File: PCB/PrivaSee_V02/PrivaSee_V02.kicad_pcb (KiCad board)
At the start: 4 copper layers, 73.8 x 90 mm, 33 parts, among them J1 RFPC-SMA27-F, J2 Batt_Solder_Point, J3 Conn_02x06_Odd_Even, J4 VOUT_TEST, J5 GND_TEST, J6 IR_TEST, J7 RF_TEST, SW1 Switch, SW2 SW_Push, U2 LM358, U3 254, U4 DFR0568, U6 ESP32-C5-DevKitC-1

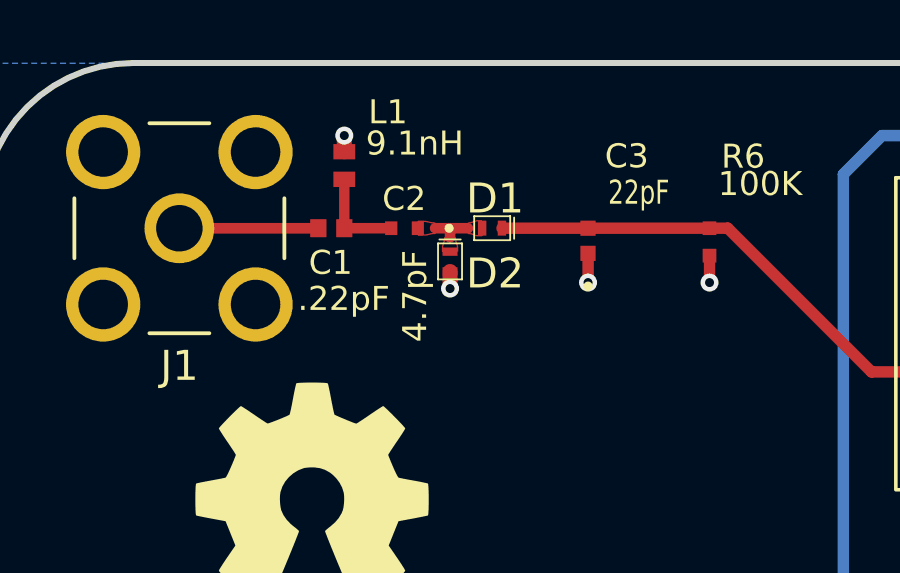
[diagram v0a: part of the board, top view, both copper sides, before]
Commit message: more trace changes
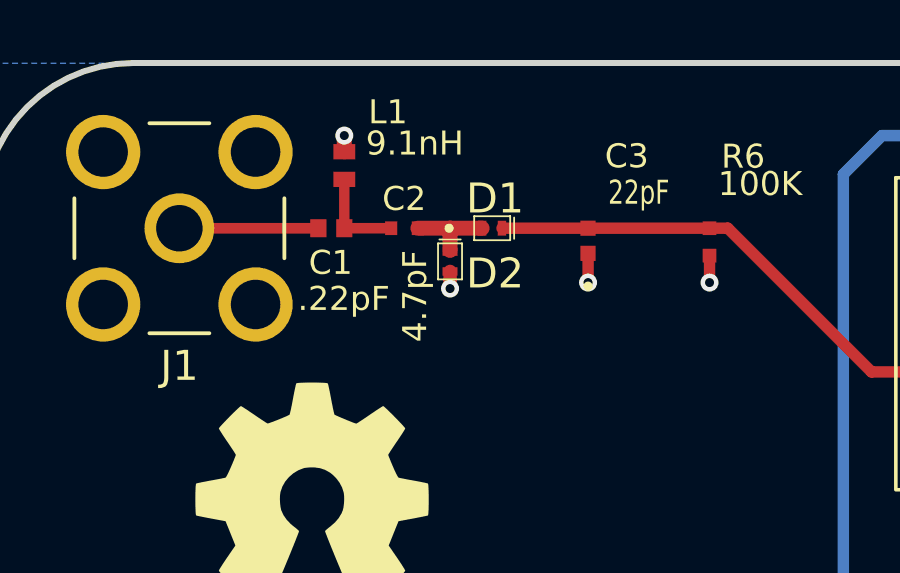
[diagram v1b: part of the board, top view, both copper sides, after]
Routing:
- net Net-(D1-A): track 1.41 -> 2.88 mm
- removed copper zone on F.Cu, net Net-(D1-A)
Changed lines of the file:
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@@
 	)
 	(segment
-		(start 81.6 27.4)
+		(start 81.6 27.0882)
+		(end 82.67 27.0882)
+		(width 0.5)
+		(layer "F.Cu")
+		(net "Net-(D1-A)")
+	)
+	(segment
+		(start 81.6 27.0882)
+		(end 81.6 27.83)
+		(width 0.5)
+		(layer "F.Cu")
+		(net "Net-(D1-A)")
+	)
+	(segment
+		(start 80.527284 27.0882)
 		(end 81.6 27.0882)
-		(width 0.35)
-		(layer "F.Cu")
-		(net "Net-(D1-A)")
-	)
-	(segment
-		(start 81.1 27.0882)
-		(end 81.6 27.0882)
-		(width 0.35)
-		(layer "F.Cu")
-		(net "Net-(D1-A)")
-	)
-	(segment
-		(start 81.6 27.0882)
-		(end 82.2 27.0882)
-		(width 0.35)
+		(width 0.5)
 		(layer "F.Cu")
 		(net "Net-(D1-A)")
@@
 		(start 81.6 29.1)
 		(end 81.6 28.53)
-		(width 0.5)
+		(width 0.45)
 		(layer "F.Cu")
 		(net "GND")
@@
 	)
 	(zone
-		(net "Net-(D1-A)")
-		(layer "F.Cu")
-		(hatch edge 0.5)
-		(priority 17540)
-		(connect_pads yes
-			(clearance 0)
-		)
-		(min_thickness 0.0254)
-		(fill yes
-			(thermal_gap 0.5)
-			(thermal_bridge_width 0.5)
-			(island_removal_mode 0)
-		)
-		(polygon
-			(pts
-				(xy 81.6 27.37375) (xy 81.425 27.3972) (xy 81.4229 27.444513) (xy 81.4172 27.48503) (xy 81.408799 27.520128)
-				(xy 81.3986 27.551189) (xy 81.3875 27.579591) (xy 81.3764 27.606713) (xy 81.3662 27.633936) (xy 81.3578 27.662638)
-				(xy 81.3521 27.6942) (xy 81.35 27.73) (xy 81.35 27.87) (xy 81.6 27.9) (xy 81.85 27.87) (xy 81.85 27.73)
-				(xy 81.8479 27.6942) (xy 81.8422 27.662638) (xy 81.833799 27.633936) (xy 81.8236 27.606713) (xy 81.8125 27.579591)
-				(xy 81.8014 27.551189) (xy 81.7912 27.520128) (xy 81.7828 27.48503) (xy 81.7771 27.444513) (xy 81.775 27.3972)
-			)
-		)
-	)
-	(zone
-		(net "Net-(D1-A)")
-		(layer "F.Cu")
-		(hatch edge 0.5)
-		(priority 17540)
-		(connect_pads yes
-			(clearance 0)
-		)
-		(min_thickness 0.0254)
-		(fill yes
-			(thermal_gap 0.5)
-			(thermal_bridge_width 0.5)
-			(island_removal_mode 0)
-		)
-		(polygon
-			(pts
-				(xy 82.17375 27.0882) (xy 82.1972 27.2632) (xy 82.244513 27.2653) (xy 82.28503 27.271) (xy 82.320128 27.279399)
-				(xy 82.351189 27.2896) (xy 82.379591 27.3007) (xy 82.406713 27.3118) (xy 82.433936 27.321999) (xy 82.462638 27.3304)
-				(xy 82.4942 27.3361) (xy 82.53 27.3382) (xy 82.67 27.3382) (xy 82.7 27.0882) (xy 82.67 26.8382)
-				(xy 82.53 26.8382) (xy 82.4942 26.8403) (xy 82.462638 26.846) (xy 82.433936 26.854399) (xy 82.406713 26.8646)
-				(xy 82.379591 26.8757) (xy 82.351189 26.8868) (xy 82.320128 26.896999) (xy 82.28503 26.9054) (xy 82.244513 26.9111)
-				(xy 82.1972 26.9132)
-			)
-		)
-	)
-	(zone
-		(net "Net-(D1-A)")
-		(layer "F.Cu")
-		(hatch edge 0.5)
-		(priority 17540)
-		(connect_pads yes
-			(clearance 0)
-		)
-		(min_thickness 0.0254)
-		(fill yes
-			(thermal_gap 0.5)
-			(thermal_bridge_width 0.5)
-			(island_removal_mode 0)
-		)
-		(polygon
-			(pts
-				(xy 81.12625 27.0882) (xy 81.104064 26.9132) (xy 81.05157 26.911699) (xy 81.006336 26.907625) (xy 80.966901 26.901622)
-				(xy 80.931804 26.894332) (xy 80.899583 26.8864) (xy 80.868777 26.878467) (xy 80.837925 26.871177)
-				(xy 80.805567 26.865174) (xy 80.77024 26.8611) (xy 80.730484 26.8596) (xy 80.527284 26.8596) (xy 80.499852 27.0882)
-				(xy 80.527284 27.3168) (xy 80.730484 27.3168) (xy 80.77024 27.315299) (xy 80.805567 27.311225) (xy 80.837925 27.305222)
-				(xy 80.868777 27.297932) (xy 80.899583 27.29) (xy 80.931804 27.282067) (xy 80.966901 27.274777)
-				(xy 81.006336 27.268774) (xy 81.05157 27.2647) (xy 81.104064 27.2632)
-			)
-		)
-	)
-	(zone
